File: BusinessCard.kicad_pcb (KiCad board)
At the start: 4 copper layers, 89 x 51 mm, 38 parts, among them J1 USB_B, U2 JW5211, U3 JW5211, U4 JW5211, U5 F1C200s, U6 W25Q80DVSNIG, Y1 24MHz

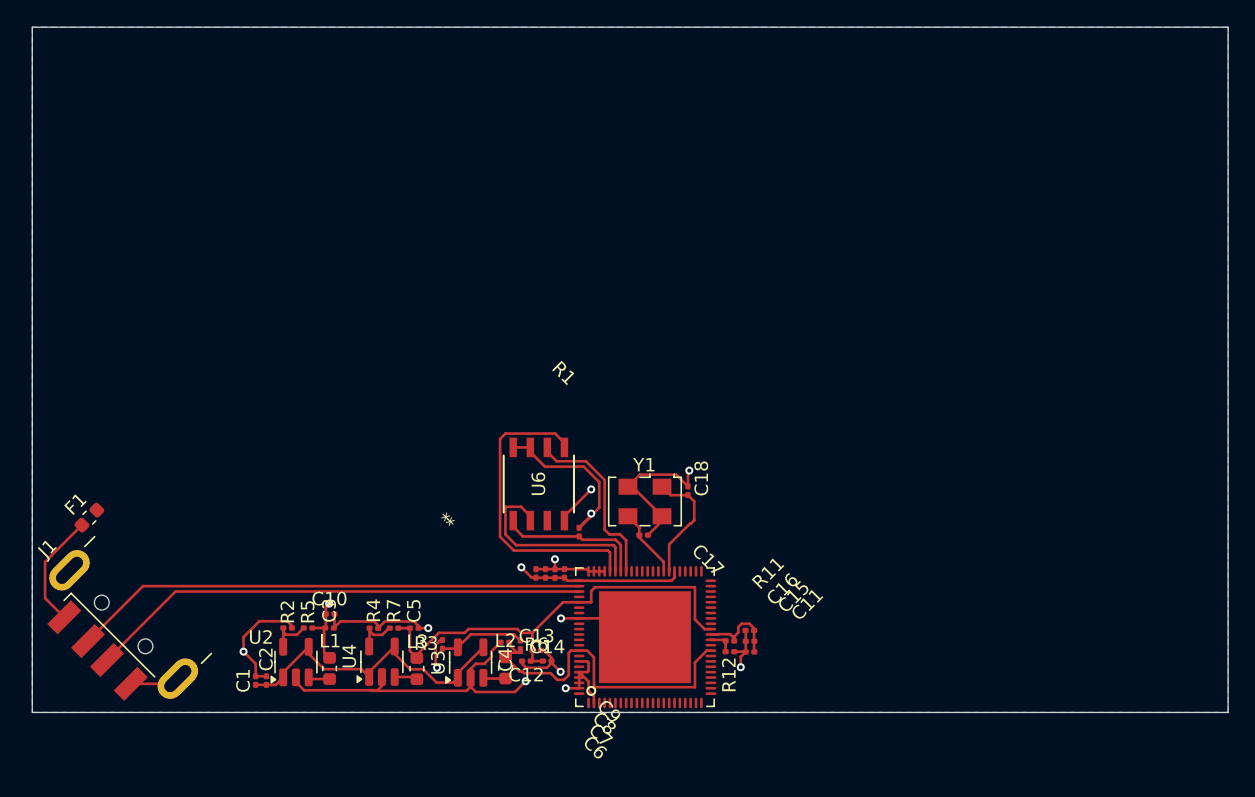
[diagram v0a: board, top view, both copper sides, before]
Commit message: progressa
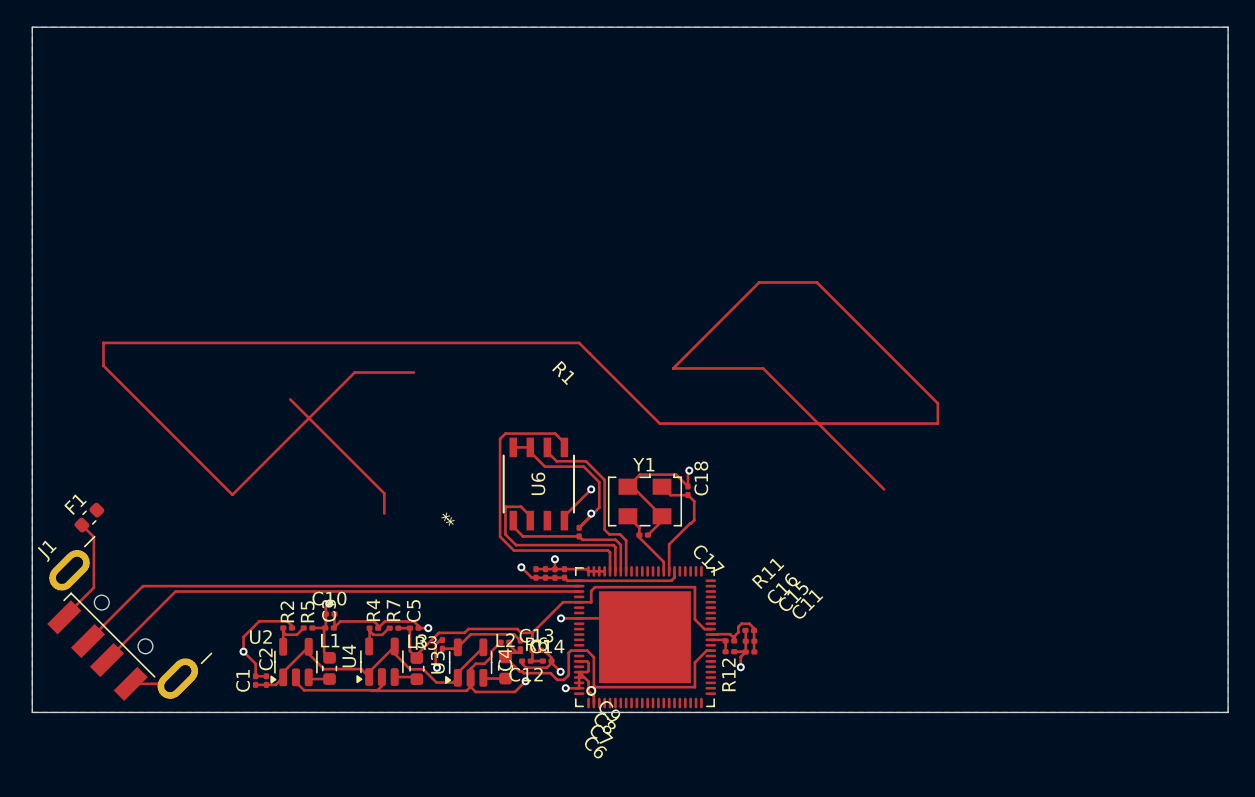
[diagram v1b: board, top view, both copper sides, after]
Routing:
- net (no net): track 0.00 -> 155.5 mm
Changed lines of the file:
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@@
+	)
+	(segment
+		(start 212.7 104.2)
+		(end 212.7 102.7)
+		(width 0.2)
+		(layer "F.Cu")
+		(net 0)
+	)
+	(segment
+		(start 191.8 91.5)
+		(end 227.2 91.5)
+		(width 0.2)
+		(layer "F.Cu")
+		(net 0)
+	)
+	(segment
+		(start 253.9 97.5)
+		(end 253.9 96)
+		(width 0.2)
+		(layer "F.Cu")
+		(net 0)
+	)
+	(segment
+		(start 233.2 97.5)
+		(end 253.9 97.5)
+		(width 0.2)
+		(layer "F.Cu")
+		(net 0)
+	)
+	(segment
+		(start 191.8 93.2)
+		(end 191.8 91.5)
+		(width 0.2)
+		(layer "F.Cu")
+		(net 0)
+	)
+	(segment
+		(start 201.4 102.8)
+		(end 191.8 93.2)
+		(width 0.2)
+		(layer "F.Cu")
+		(net 0)
+	)
+	(segment
+		(start 240.9 93.4)
+		(end 249.9 102.4)
+		(width 0.2)
+		(layer "F.Cu")
+		(net 0)
+	)
+	(segment
+		(start 253.9 96)
+		(end 244.9 87)
+		(width 0.2)
+		(layer "F.Cu")
+		(net 0)
+	)
+	(segment
+		(start 227.2 91.5)
+		(end 228 92.3)
+		(width 0.2)
+		(layer "F.Cu")
+		(net 0)
+	)
+	(segment
+		(start 214.9 93.7)
+		(end 210.5 93.7)
+		(width 0.2)
+		(layer "F.Cu")
+		(net 0)
+	)
+	(segment
+		(start 228 92.3)
+		(end 233.2 97.5)
+		(width 0.2)
+		(layer "F.Cu")
+		(net 0)
+	)
+	(segment
+		(start 234.2 93.4)
+		(end 240.9 93.4)
+		(width 0.2)
+		(layer "F.Cu")
+		(net 0)
+	)
+	(segment
+		(start 244.9 87)
+		(end 240.6 87)
+		(width 0.2)
+		(layer "F.Cu")
+		(net 0)
+	)
+	(segment
+		(start 212.7 102.7)
+		(end 205.7 95.7)
+		(width 0.2)
+		(layer "F.Cu")
+		(net 0)
+	)
+	(segment
+		(start 240.6 87)
+		(end 234.2 93.4)
+		(width 0.2)
+		(layer "F.Cu")
+		(net 0)
+	)
+	(segment
+		(start 210.5 93.7)
+		(end 201.4 102.8)
+		(width 0.2)
+		(layer "F.Cu")
+		(net 0)
 	)
 	(segment
@@
 	)
 	(segment
-		(start 187.452014 107.797986)
-		(end 190.193153 105.056847)
+		(start 191.083384 109.71687)
+		(end 188.87879 111.921464)
 		(width 0.2)
 		(layer "F.Cu")
@@
 	)
 	(segment
-		(start 187.452014 110.494688)
-		(end 187.452014 107.797986)
+		(start 190.193153 105.056847)
+		(end 191.083384 105.947078)
 		(width 0.2)
 		(layer "F.Cu")
@@
 	)
 	(segment
-		(start 188.87879 111.921464)
-		(end 187.452014 110.494688)
-		(width 0.2)
-		(layer "F.Cu")
+		(start 191.083384 105.947078)
+		(end 191.083384 109.71687)
+		(width 0.2)
+		(layer "F.Cu")
